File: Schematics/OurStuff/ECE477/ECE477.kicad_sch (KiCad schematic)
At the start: 30 parts, among them J1 USB_B_Micro, J2 Barrel_Jack, Q1 SS8050-G, Q2 SS8050-G, SW1 SW_Push, SW2 SW_Push, U1 ESP32-WROOM-32E, U2 CP2102N-Axx-xQFN28

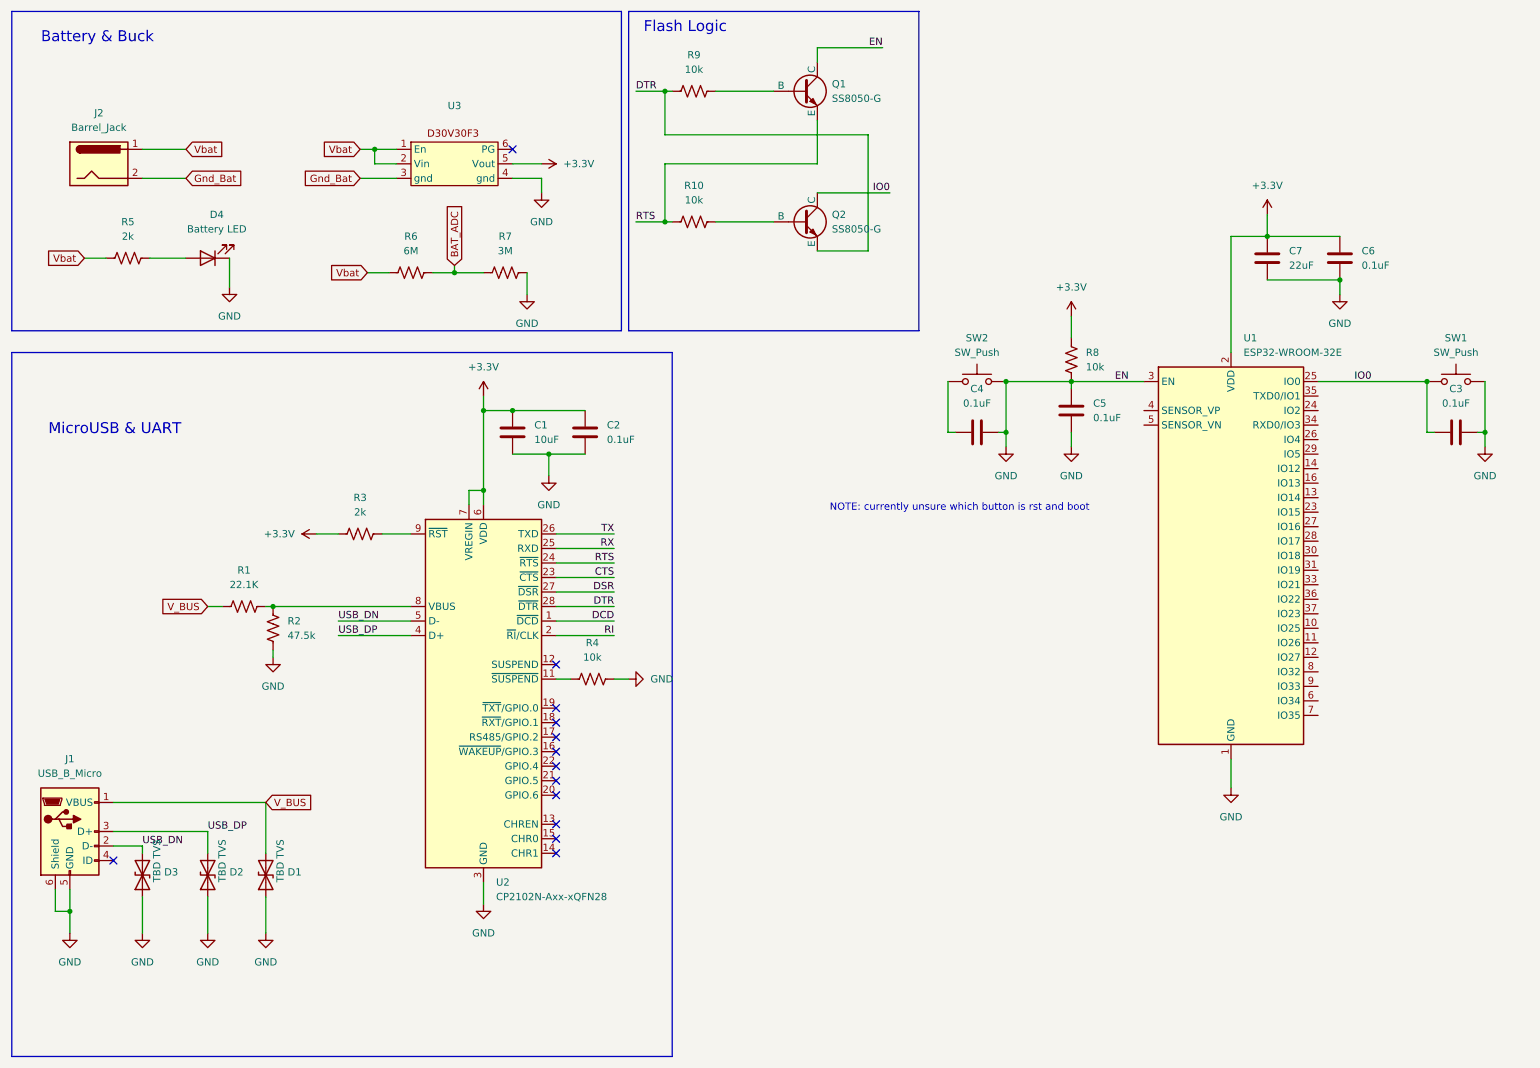
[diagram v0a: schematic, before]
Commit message: Added Peripherals
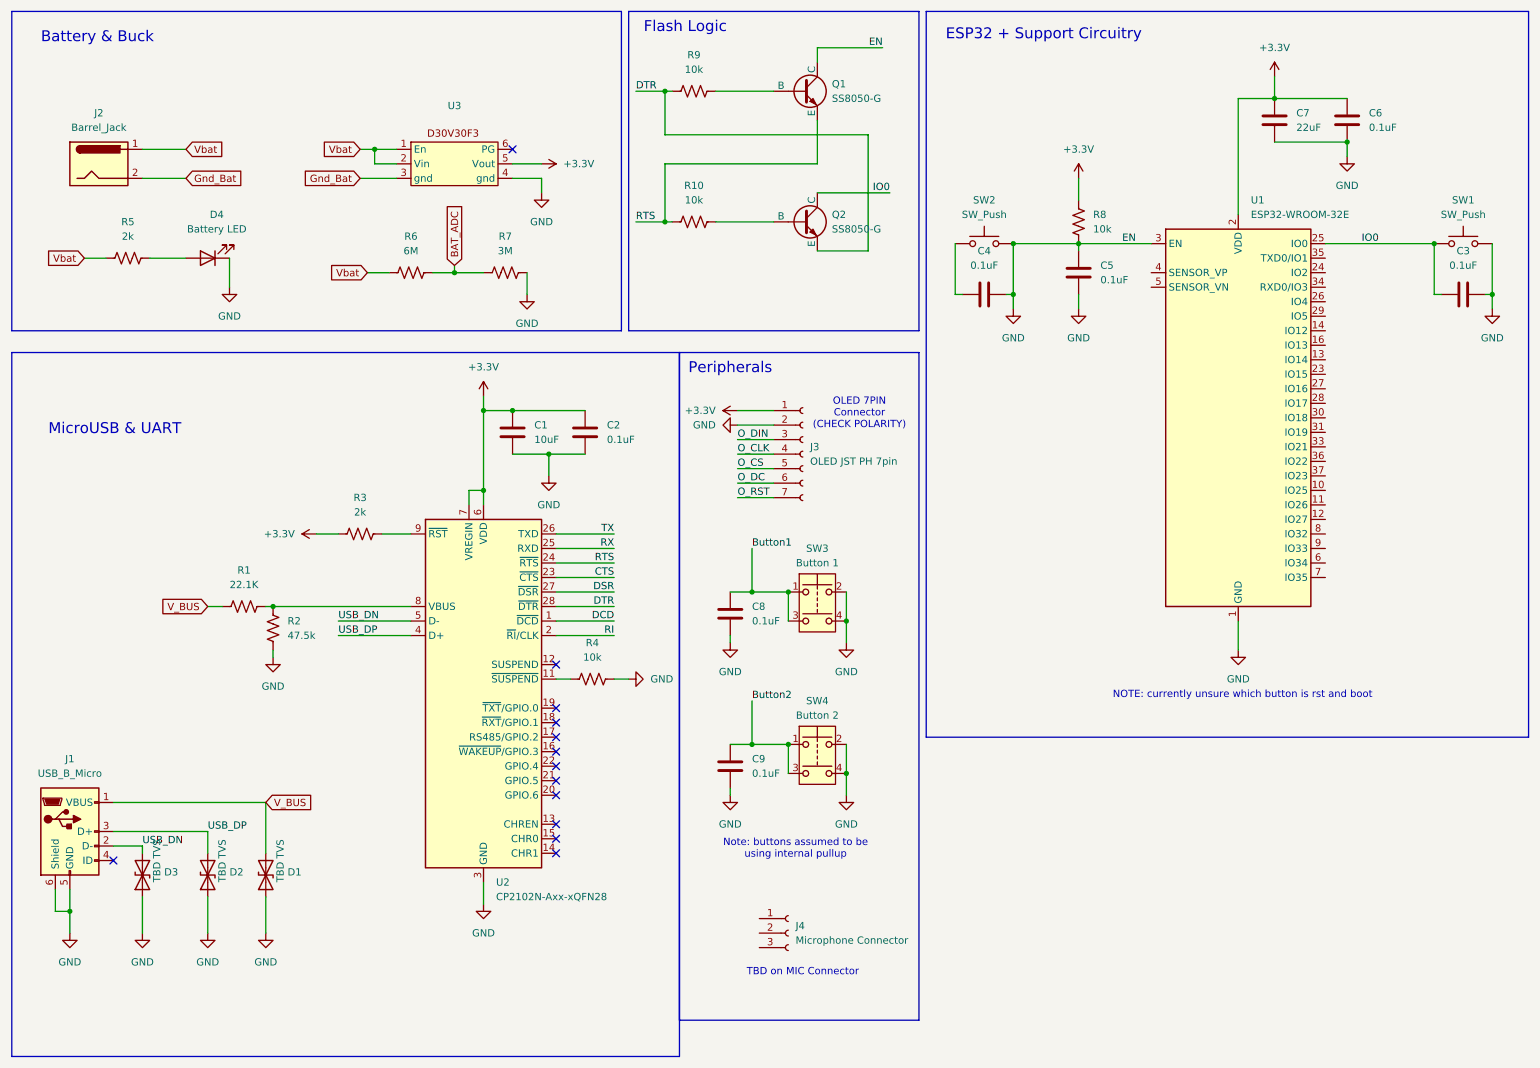
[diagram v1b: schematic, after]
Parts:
- added C8, C9: 0.1uF, symbol Device:C
- added J3: OLED JST PH 7pin, symbol Connector:Conn_01x07_Socket
- added J4: Microphone Connector, symbol Connector:Conn_01x03_Socket
- added SW3: Button 1, symbol Switch:SW_Push_Dual
- added SW4: Button 2, symbol Switch:SW_Push_Dual
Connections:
- net +3.3V: now also J3.1 (Pin_1)
- net GND: now also C8.2, C9.2, J3.2 (Pin_2), SW3.2, SW3.4, SW4.2, SW4.4
- new net Button1: C8.1, SW3.1, SW3.3
- new net Button2: C9.1, SW4.1, SW4.3
- new net O_CLK: J3.4 (Pin_4)
- new net O_CS: J3.5 (Pin_5)
- new net O_DC: J3.6 (Pin_6)
- new net O_DIN: J3.3 (Pin_3)
- new net O_RST: J3.7 (Pin_7)
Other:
- note added: "ESP32 + Support Circuitry"
- note added: "Note: buttons assumed to be using internal pullup"
- note added: "OLED 7PIN Connector (CHECK POLARITY)"
- note added: "Peripherals"
- note added: "TBD on MIC Connector"
- moved on the sheet: C3, C4, C5, C6, C7, R8, SW1, SW2, U1

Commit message: added debug
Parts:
- removed C5: 0.1uF, symbol Device:C
- added D5: Power LED, symbol Device:LED
- added D6: TX_LED, symbol Device:LED
- added D7, D8, D9: RX_LED, symbol Device:LED
- added J5, J6: Conn_01x02_Pin, symbol Connector:Conn_01x02_Pin
- added R11, R12: 10k, symbol Device:R_US
- added R13, R15, R16, R17, R18: 220, symbol Device:R_US
- D1, D2, D3: value TBD TVS -> ESD9B5.0ST5G
- SW1: value SW_Push -> Boot Button
- SW2: value SW_Push -> RST Button
- U3: value ~ -> D30V30F3
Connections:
- net +3.3V: now also J4.3 (Pin_3), R11.1, R12.1, R13.1
- net Button1: now also R11.2
- net Button2: now also R12.2
- net GND: now also C4.2, J4.2 (Pin_2), SW2.1, D5.1 (K), D6.1 (K), D7.1 (K), D8.1 (K), D9.1 (K); no longer C4.1, J1.6 (Shield), Q1.1 (C), R8.1, SW2.2, U1.3 (EN)
- net O_CLK: now also U1.30 (IO18)
- net O_CS: now also U1.33 (IO21)
- net O_DC: now also U1.31 (IO19)
- net O_DIN: now also U1.37 (IO23)
- net O_RST: now also U1.36 (IO22)
- net RX: now also U1.34 (RXD0/IO3), J5.2 (Pin_2), R16.1
- net TX: now also U1.35 (TXD0/IO1), J5.1 (Pin_1), R15.1
- net Vbat: now also U1.4 (SENSOR_VP)
- net Mic_In: now reaches J4.1 (Pin_1)
- net Mic_In: now also U1.6 (IO34)
- net Debug_1: now reaches U1.10 (IO25)
- net Debug_1: now also R17.1
- net Debug_2: now reaches U1.11 (IO26)
- net Debug_2: now also R18.1
- net Debug_3: now reaches U1.12 (IO27)
- net Debug_3: now also J6.1 (Pin_1)
- net Debug_4: now reaches U1.8 (IO32)
- net Debug_4: now also J6.2 (Pin_2)
- net CTS: no longer names the net of U2.23 (~{CTS})
- net DCD: no longer names the net of U2.1 (~{DCD})
- net DSR: no longer names the net of U2.27 (~{DSR})
- net RI: no longer names the net of U2.2 (~{RI}/CLK)
- new net: D5.2 (A), R13.2
- new net: D8.2 (A), R17.2
- new net: D7.2 (A), R16.2
- new net: D6.2 (A), R15.2
- new net: D9.2 (A), R18.2
- new net EN: C4.1, Q1.1 (C), R8.1, SW2.2, U1.3 (EN)
- no-connect marks 13 -> 30
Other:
- note added: "Buttons"
- note added: "General DEBUG"
- note added: "Note: assume gpio0-gpio17 are special and should not have anything attatched to them"
- note added: "Note: assuming the debug connectors are just header pins"
- note added: "UART DEBUG"
- note removed: "NOTE: currently unsure which button is rst and boot"
- note removed: "Note: buttons assumed to be using internal pullup"
- moved on the sheet: C1, C2, C4, C6, C7, C8, C9, D1, D2, D3, D4, J1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
